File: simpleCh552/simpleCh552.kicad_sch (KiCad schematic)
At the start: 14 parts, among them J1 A0, J2 A1, J3 A2, J4 A3, J5 Conn_01x04, SW1 SW_SPST, U1 CH552G

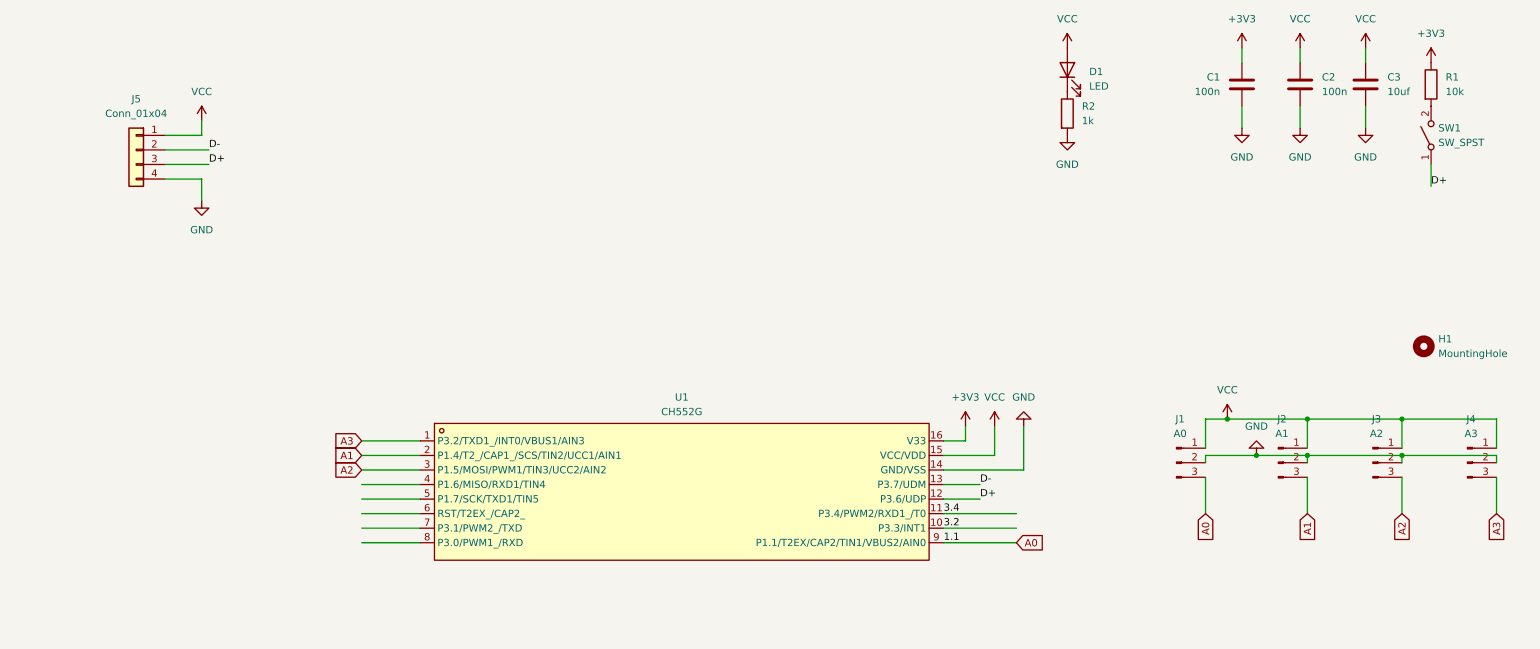
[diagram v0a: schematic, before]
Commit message: update
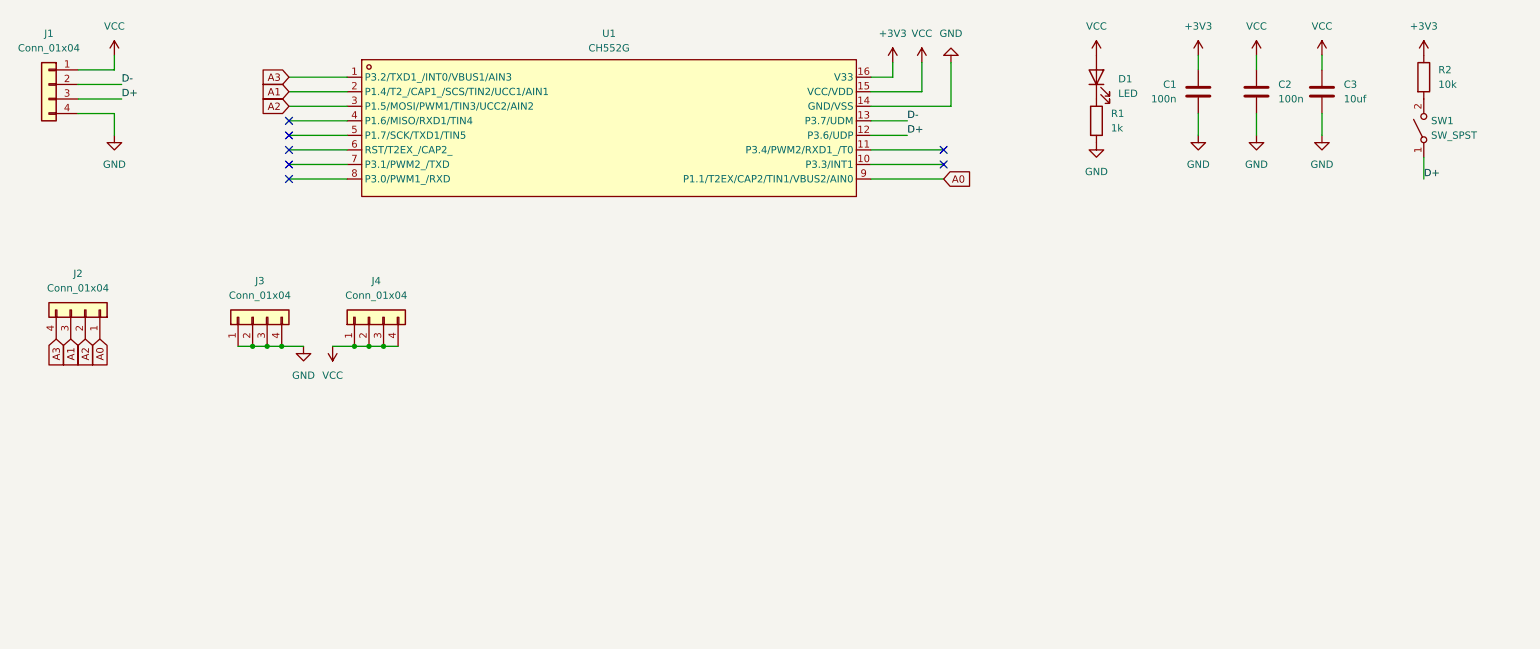
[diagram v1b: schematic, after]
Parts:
- removed H1: MountingHole, MountingHole:MountingHole_2.1mm, symbol Mechanical:MountingHole
- removed J1: A0, Connector_PinSocket_2.00mm:PinSocket_1x03_P2.00mm_Vertical, symbol Connector:Conn_01x03_Pin
- removed J2: A1, Connector_PinSocket_2.00mm:PinSocket_1x03_P2.00mm_Vertical, symbol Connector:Conn_01x03_Pin
- removed J3: A2, Connector_PinSocket_2.00mm:PinSocket_1x03_P2.00mm_Vertical, symbol Connector:Conn_01x03_Pin
- removed J4: A3, Connector_PinSocket_2.00mm:PinSocket_1x03_P2.00mm_Vertical, symbol Connector:Conn_01x03_Pin
- added J2, J3, J4: Conn_01x04, Connector_Wire:SolderWire-0.5sqmm_1x04_P4.6mm_D0.9mm_OD2.1mm, symbol Connector_Generic:Conn_01x04
- renumbered J5 to J1, R2 to R1, R1 to R2
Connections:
- net A0: now also J2.1 (Pin_1)
- net A1: now also J2.3 (Pin_3)
- net A2: now also J2.2 (Pin_2)
- net A3: now also J2.4 (Pin_4)
- net GND: now also J3.1 (Pin_1), J3.2 (Pin_2), J3.3 (Pin_3), J3.4 (Pin_4)
- net VCC: now also J4.1 (Pin_1), J4.2 (Pin_2), J4.3 (Pin_3), J4.4 (Pin_4)
- net 3.2: no longer names the net of U1.10 (P3.3/INT1)
- net 3.4: no longer names the net of U1.11 (P3.4/PWM2/RXD1_/T0)
- no-connect marks 0 -> 7
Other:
- moved on the sheet: C1, C2, C3, D1, J1, R1, R2, SW1, U1

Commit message: updated with pot
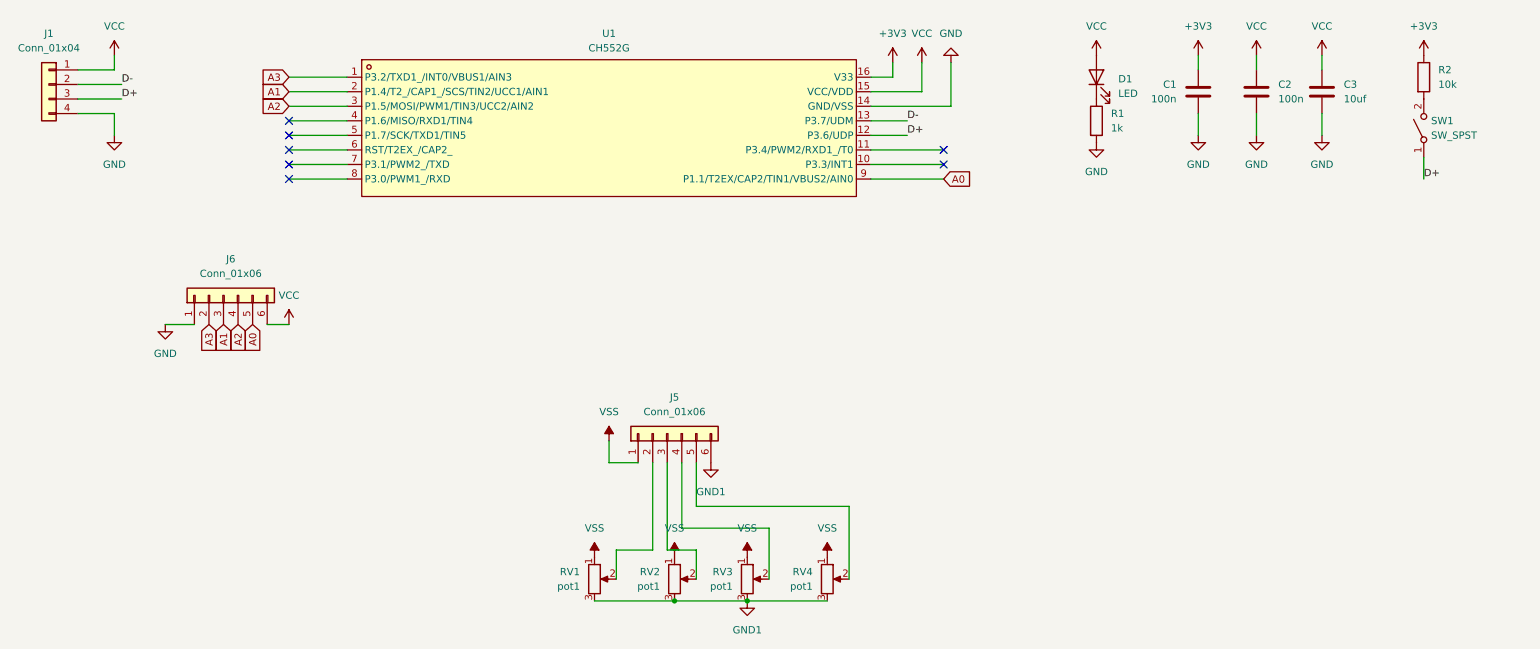
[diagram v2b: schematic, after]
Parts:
- removed J2, J3, J4: Conn_01x04, Connector_Wire:SolderWire-0.5sqmm_1x04_P4.6mm_D0.9mm_OD2.1mm, symbol Connector_Generic:Conn_01x04
- added J5, J6: Conn_01x06, Connector_Wire:SolderWire-0.1sqmm_1x06_P3.6mm_D0.4mm_OD1mm, symbol Connector_Generic:Conn_01x06
- added RV1, RV2, RV3, RV4: pot1, Potentiometer_THT:Potentiometer_Omeg_PC16BU_Vertical, symbol Device:R_Potentiometer
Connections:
- net A0: now also J6.5 (Pin_5)
- net A1: now also J6.3 (Pin_3)
- net A2: now also J6.4 (Pin_4)
- net A3: now also J6.2 (Pin_2)
- net GND: now also J6.1 (Pin_1)
- net VCC: now also J6.6 (Pin_6)
- new net: J5.5 (Pin_5), RV4.2
- new net: J5.4 (Pin_4), RV3.2
- new net: J5.3 (Pin_3), RV2.2
- new net: J5.2 (Pin_2), RV1.2
- new net GND1: J5.6 (Pin_6), RV1.3, RV2.3, RV3.3, RV4.3
- new net VSS: J5.1 (Pin_1), RV1.1, RV2.1, RV3.1, RV4.1
